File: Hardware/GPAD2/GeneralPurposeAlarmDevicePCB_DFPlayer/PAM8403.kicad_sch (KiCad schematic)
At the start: 2 parts

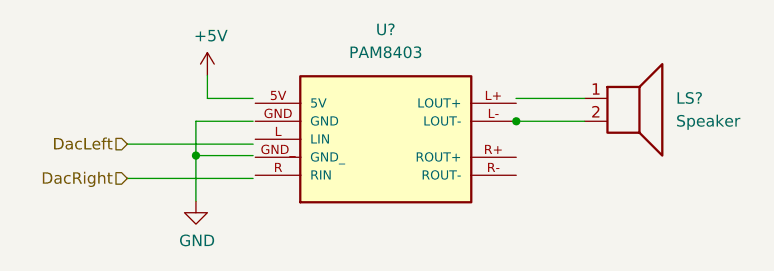
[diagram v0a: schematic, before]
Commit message: updated hardware
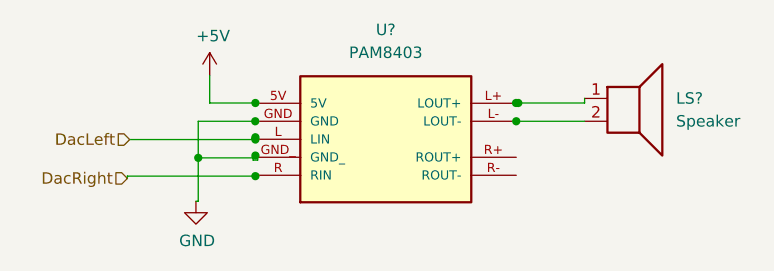
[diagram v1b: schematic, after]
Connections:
- net GND: now also U?.GND
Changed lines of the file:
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@@
 (kicad_sch (version 20211123) (generator eeschema)
   (paper "A4")
-  (junction (at 125.73 93.98) (diameter 0) (color 0 0 0 0)
+  (junction (at 132.334 96.266) (diameter 0) (color 0 0 0 0)
+  )
+  (junction (at 132.32 90.17) (diameter 0) (color 0 0 0 0)
+  )
+  (junction (at 132.334 92.202) (diameter 0) (color 0 0 0 0)
+  )
+  (junction (at 132.334 91.948) (diameter 0) (color 0 0 0 0)
+  )
+  (junction (at 132.334 93.98) (diameter 0) (color 0 0 0 0)
+  )
+  (junction (at 161.544 88.138) (diameter 0) (color 0 0 0 0)
   )
   (junction (at 161.32 90.17) (diameter 0) (color 0 0 0 0)
   )
-  (wire (pts (xy 127 87.63) (xy 127 85.09))
-    (stroke (width 0) (type default) (color 0 0 0 0))
-  )
-  (wire (pts (xy 125.73 93.98) (xy 132.08 93.98))
-    (stroke (width 0) (type default) (color 0 0 0 0))
-  )
-  (wire (pts (xy 132.08 90.17) (xy 125.73 90.17))
-    (stroke (width 0) (type default) (color 0 0 0 0))
-  )
-  (wire (pts (xy 118.11 92.71) (xy 132.08 92.71))
+  (junction (at 125.984 94.234) (diameter 0) (color 0 0 0 0)
+  )
+  (junction (at 161.29 88.138) (diameter 0) (color 0 0 0 0)
+  )
+  (junction (at 132.334 88.138) (diameter 0) (color 0 0 0 0)
+  )
+  (wire (pts (xy 161.29 88.392) (xy 161.544 88.392))
+    (stroke (width 0) (type default) (color 0 0 0 0))
+  )
+  (wire (pts (xy 132.334 93.98) (xy 132.588 93.98))
+    (stroke (width 0) (type default) (color 0 0 0 0))
+  )
+  (wire (pts (xy 127.254 88.138) (xy 127.254 85.09))
+    (stroke (width 0) (type default) (color 0 0 0 0))
+  )
+  (wire (pts (xy 161.29 87.884) (xy 161.29 88.138))
+    (stroke (width 0) (type default) (color 0 0 0 0))
+  )
+  (wire (pts (xy 132.08 88.392) (xy 132.334 88.392))
+    (stroke (width 0) (type default) (color 0 0 0 0))
+  )
+  (wire (pts (xy 132.334 92.202) (xy 132.334 92.456))
+    (stroke (width 0) (type default) (color 0 0 0 0))
+  )
+  (wire (pts (xy 132.334 91.948) (xy 132.334 92.202))
+    (stroke (width 0) (type default) (color 0 0 0 0))
+  )
+  (wire (pts (xy 132.588 93.98) (xy 132.588 94.488))
+    (stroke (width 0) (type default) (color 0 0 0 0))
+  )
+  (wire (pts (xy 132.08 93.98) (xy 132.334 93.98))
+    (stroke (width 0) (type default) (color 0 0 0 0))
+  )
+  (wire (pts (xy 161.544 88.392) (xy 161.544 88.138))
+    (stroke (width 0) (type default) (color 0 0 0 0))
+  )
+  (wire (pts (xy 125.984 94.234) (xy 125.984 99.06))
+    (stroke (width 0) (type default) (color 0 0 0 0))
+  )
+  (wire (pts (xy 161.29 88.138) (xy 161.29 88.392))
+    (stroke (width 0) (type default) (color 0 0 0 0))
+  )
+  (wire (pts (xy 125.984 90.17) (xy 132.32 90.17))
+    (stroke (width 0) (type default) (color 0 0 0 0))
+  )
+  (wire (pts (xy 132.588 91.948) (xy 132.588 92.202))
+    (stroke (width 0) (type default) (color 0 0 0 0))
+  )
+  (wire (pts (xy 161.544 88.138) (xy 168.91 88.138))
+    (stroke (width 0) (type default) (color 0 0 0 0))
+  )
+  (wire (pts (xy 132.08 91.948) (xy 132.334 91.948))
+    (stroke (width 0) (type default) (color 0 0 0 0))
+  )
+  (wire (pts (xy 125.984 94.234) (xy 132.334 94.234))
+    (stroke (width 0) (type default) (color 0 0 0 0))
+  )
+  (wire (pts (xy 132.588 88.138) (xy 132.334 88.138))
+    (stroke (width 0) (type default) (color 0 0 0 0))
+  )
+  (wire (pts (xy 132.334 96.012) (xy 132.588 96.012))
+    (stroke (width 0) (type default) (color 0 0 0 0))
+  )
+  (wire (pts (xy 132.32 90.17) (xy 132.334 90.17))
+    (stroke (width 0) (type default) (color 0 0 0 0))
+  )
+  (wire (pts (xy 132.334 96.52) (xy 132.334 96.266))
     (stroke (width 0) (type default) (color 0 0 0 0))
   )
@@
     (stroke (width 0) (type default) (color 0 0 0 0))
   )
+  (wire (pts (xy 125.984 90.17) (xy 125.984 94.234))
+    (stroke (width 0) (type default) (color 0 0 0 0))
+  )
+  (wire (pts (xy 132.588 94.488) (xy 132.08 94.488))
+    (stroke (width 0) (type default) (color 0 0 0 0))
+  )
   (wire (pts (xy 161.29 90.17) (xy 161.32 90.17))
     (stroke (width 0) (type default) (color 0 0 0 0))
   )
-  (wire (pts (xy 118.11 96.52) (xy 132.08 96.52))
-    (stroke (width 0) (type default) (color 0 0 0 0))
-  )
-  (wire (pts (xy 125.73 90.17) (xy 125.73 93.98))
-    (stroke (width 0) (type default) (color 0 0 0 0))
-  )
-  (wire (pts (xy 127 87.63) (xy 132.08 87.63))
-    (stroke (width 0) (type default) (color 0 0 0 0))
-  )
-  (wire (pts (xy 161.29 87.63) (xy 168.91 87.63))
-    (stroke (width 0) (type default) (color 0 0 0 0))
-  )
-  (wire (pts (xy 125.73 93.98) (xy 125.73 99.06))
-    (stroke (width 0) (type default) (color 0 0 0 0))
-  )
-  (hierarchical_label "DacLeft" (shape input) (at 118.11 92.71 180)
+  (wire (pts (xy 132.588 92.202) (xy 132.334 92.202))
+    (stroke (width 0) (type default) (color 0 0 0 0))
+  )
+  (wire (pts (xy 132.08 94.488) (xy 132.08 93.98))
+    (stroke (width 0) (type default) (color 0 0 0 0))
+  )
+  (wire (pts (xy 132.334 96.266) (xy 118.11 96.266))
+    (stroke (width 0) (type default) (color 0 0 0 0))
+  )
+  (wire (pts (xy 132.334 91.948) (xy 132.588 91.948))
+    (stroke (width 0) (type default) (color 0 0 0 0))
+  )
+  (wire (pts (xy 132.334 96.266) (xy 132.334 96.012))
+    (stroke (width 0) (type default) (color 0 0 0 0))
+  )
+  (wire (pts (xy 132.334 88.138) (xy 132.334 88.392))
+    (stroke (width 0) (type default) (color 0 0 0 0))
+  )
+  (wire (pts (xy 127.254 88.138) (xy 132.334 88.138))
+    (stroke (width 0) (type default) (color 0 0 0 0))
+  )
+  (wire (pts (xy 161.29 88.138) (xy 161.544 88.138))
+    (stroke (width 0) (type default) (color 0 0 0 0))
+  )
+  (wire (pts (xy 118.364 92.202) (xy 132.334 92.202))
+    (stroke (width 0) (type default) (color 0 0 0 0))
+  )
+  (wire (pts (xy 118.11 96.266) (xy 118.11 96.52))
+    (stroke (width 0) (type default) (color 0 0 0 0))
+  )
+  (wire (pts (xy 132.588 96.266) (xy 132.334 96.266))
+    (stroke (width 0) (type default) (color 0 0 0 0))
+  )
+  (wire (pts (xy 132.588 96.012) (xy 132.588 96.266))
+    (stroke (width 0) (type default) (color 0 0 0 0))
+  )
+  (wire (pts (xy 132.334 93.98) (xy 132.334 94.234))
+    (stroke (width 0) (type default) (color 0 0 0 0))
+  )
+  (wire (pts (xy 125.984 99.06) (xy 125.73 99.06))
+    (stroke (width 0) (type default) (color 0 0 0 0))
+  )
+  (wire (pts (xy 132.334 87.884) (xy 132.334 88.138))
+    (stroke (width 0) (type default) (color 0 0 0 0))
+  )
+  (wire (pts (xy 168.91 88.138) (xy 168.91 87.63))
+    (stroke (width 0) (type default) (color 0 0 0 0))
+  )
+  (hierarchical_label "DacLeft" (shape input) (at 118.364 92.202 180)
     (effects (font (size 1.27 1.27)) (justify right))
   )
@@
     (pin "1")
   )
-  (symbol (lib_id "power:+5V") (at 127 85.09 0) (unit 1)
+  (symbol (lib_id "power:+5V") (at 127.254 85.09 0) (unit 1)
     (in_bom yes) (on_board yes)
-    (property "Reference" "#PWR?" (id 0) (at 127 88.9 0)
-      (effects (font (size 1.27 1.27)) hide)
-    )
-    (property "Value" "+5V" (id 1) (at 127.381 80.6958 0))
-    (property "Footprint" "" (id 2) (at 127 85.09 0)
-      (effects (font (size 1.27 1.27)) hide)
-    )
-    (property "Datasheet" "" (id 3) (at 127 85.09 0)
-      (effects (font (size 1.27 1.27)) hide)
-    )
+    (property "Reference" "#PWR?" (id 0) (at 127.254 88.9 0)
+      (effects (font (size 1.27 1.27)) hide)
+    )
+    (property "Value" "+5V" (id 1) (at 127.635 80.6958 0))
+    (property "Footprint" "" (id 2) (at 127.254 85.09 0)
+      (effects (font (size 1.27 1.27)) hide)
+    )
+    (property "Datasheet" "" (id 3) (at 127.254 85.09 0)
+      (effects (font (size 1.27 1.27)) hide)
+    )
